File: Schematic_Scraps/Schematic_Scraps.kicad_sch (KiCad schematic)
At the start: 1 part, among them U5 8080A

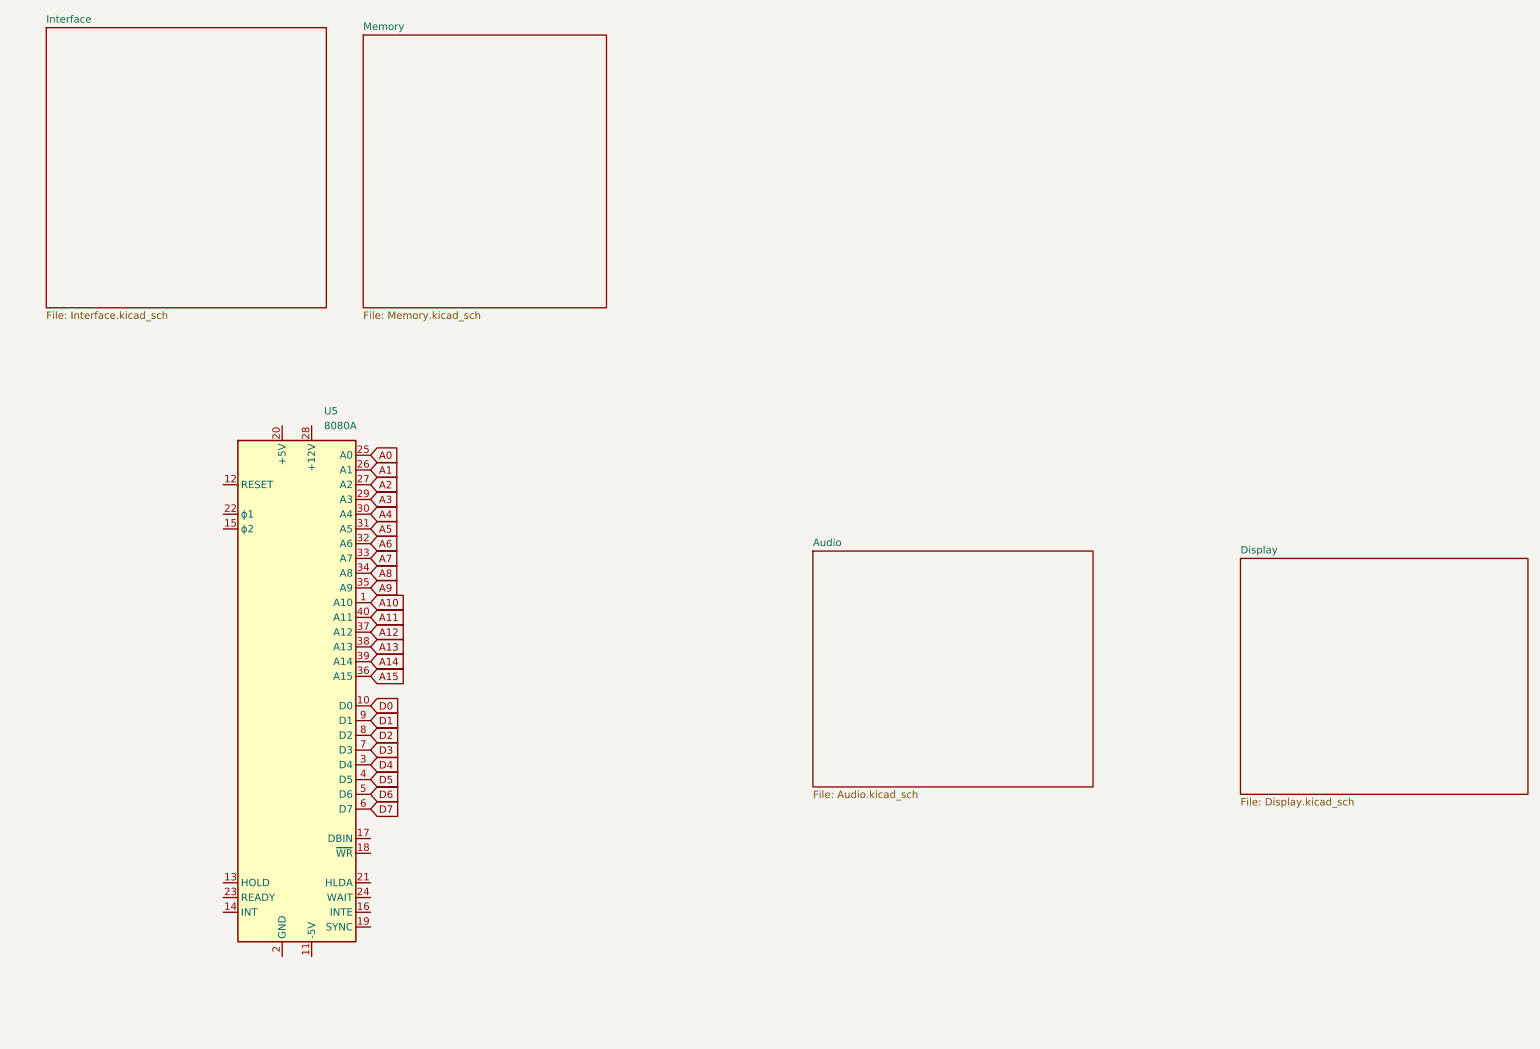
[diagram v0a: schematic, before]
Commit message: Further reverse engineering progress
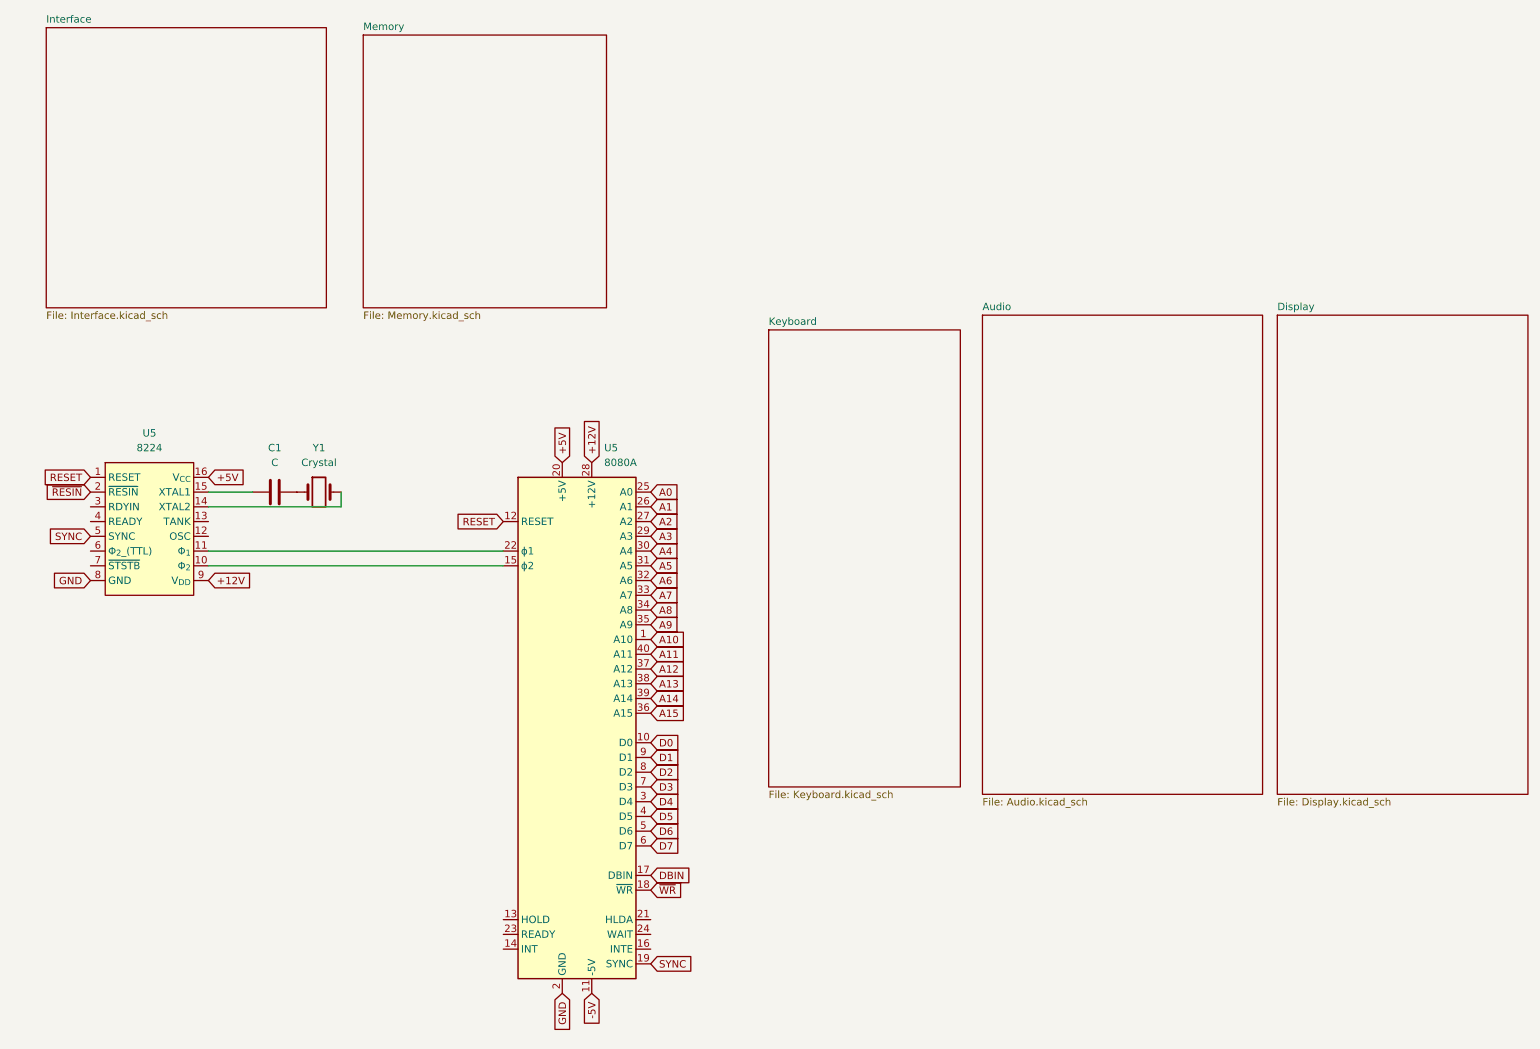
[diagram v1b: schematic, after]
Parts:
- added C1: C, symbol Device:C
- added U5: 8224, Package_DIP:DIP-16_W7.62mm, symbol Clueless_Engineer:8224
- added Y1: Crystal, symbol Device:Crystal
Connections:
- net -5V: now reaches U5.11 (-5V)
- net RESET: now reaches U5.12 (RESET)
- net RESET: now also U5.1 (RESET)
- net at U5.15 (ϕ2): now also U5.10 (Φ_{2})
- net DBIN: now reaches U5.17 (DBIN)
- net ~{WR}: now reaches U5.18 (~{WR})
- net SYNC: now reaches U5.19 (SYNC)
- net SYNC: now also U5.5 (SYNC)
- net GND: now reaches U5.2 (GND)
- net GND: now also U5.8 (GND)
- net +5V: now reaches U5.20 (+5V)
- net +5V: now also U5.16 (V_{CC})
- net at U5.22 (ϕ1): now also U5.11 (Φ_{1})
- net +12V: now reaches U5.28 (+12V)
- net +12V: now also U5.9 (V_{DD})
- new net: C1.1, U5.15 (XTAL1)
- new net: C1.2, Y1.1
- new net: U5.14 (XTAL2), Y1.2
- new net ~{RESIN}: U5.2 (~{RESIN})
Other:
- added sheet Keyboard (Keyboard.kicad_sch)
- company: (none) -> Brett Hallen
- title: (none) -> Rhythm Keyboard (Ритм Клав)
- moved on the sheet: U5
